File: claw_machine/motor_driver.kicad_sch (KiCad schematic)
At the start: 3 parts, among them J3 Screw_Terminal_01x02, J4 Screw_Terminal_01x02, U1 L298N

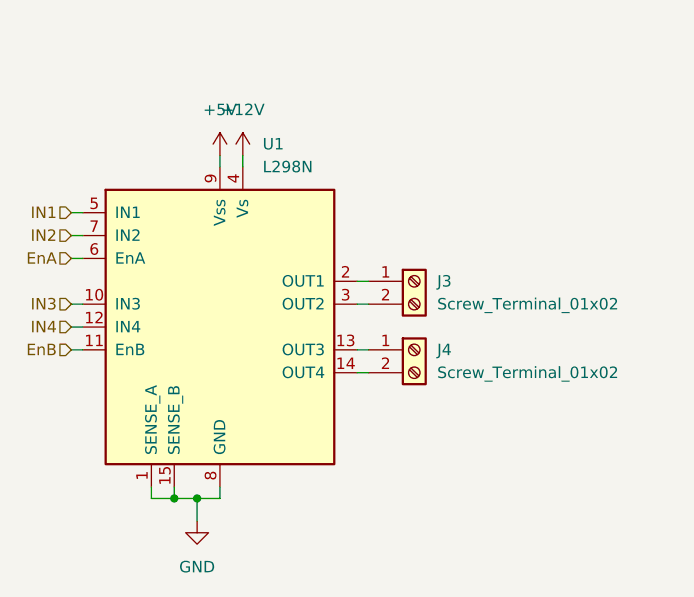
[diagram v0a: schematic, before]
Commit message: change folder stuff & update gen pwr
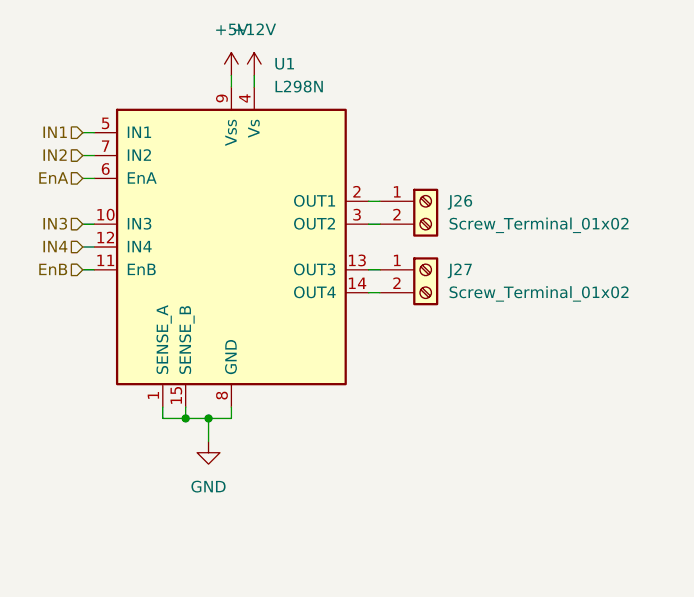
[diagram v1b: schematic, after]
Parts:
- removed J3, J4: Screw_Terminal_01x02, symbol Connector:Screw_Terminal_01x02
- added J26, J27: Screw_Terminal_01x02, TerminalBlock:TerminalBlock_bornier-2_P5.08mm, symbol Connector:Screw_Terminal_01x02
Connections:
- net at U1.13 (OUT3): now also J27.1 (Pin_1)
- net at U1.14 (OUT4): now also J27.2 (Pin_2)
- net at U1.2 (OUT1): now also J26.1 (Pin_1)
- net at U1.3 (OUT2): now also J26.2 (Pin_2)
